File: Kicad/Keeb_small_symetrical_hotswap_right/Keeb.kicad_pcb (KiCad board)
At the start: 2 copper layers, 96.3 x 99.3 mm, 28 parts, among them J1 TYPE-C-31-M-12, SW1 CherryMX, SW10 CherryMX, SW11 CherryMX, SW13 CherryMX, SW14 CherryMX, SW15 CherryMX, SW16 CherryMX, SW17 CherryMX, SW18 CherryMX, SW19 CherryMX, SW20 CherryMX, SW3 CherryMX, SW4 CherryMX, SW5 CherryMX, SW6 CherryMX, SW7 CherryMX, SW8 CherryMX, SW9 CherryMX, U1 Pico

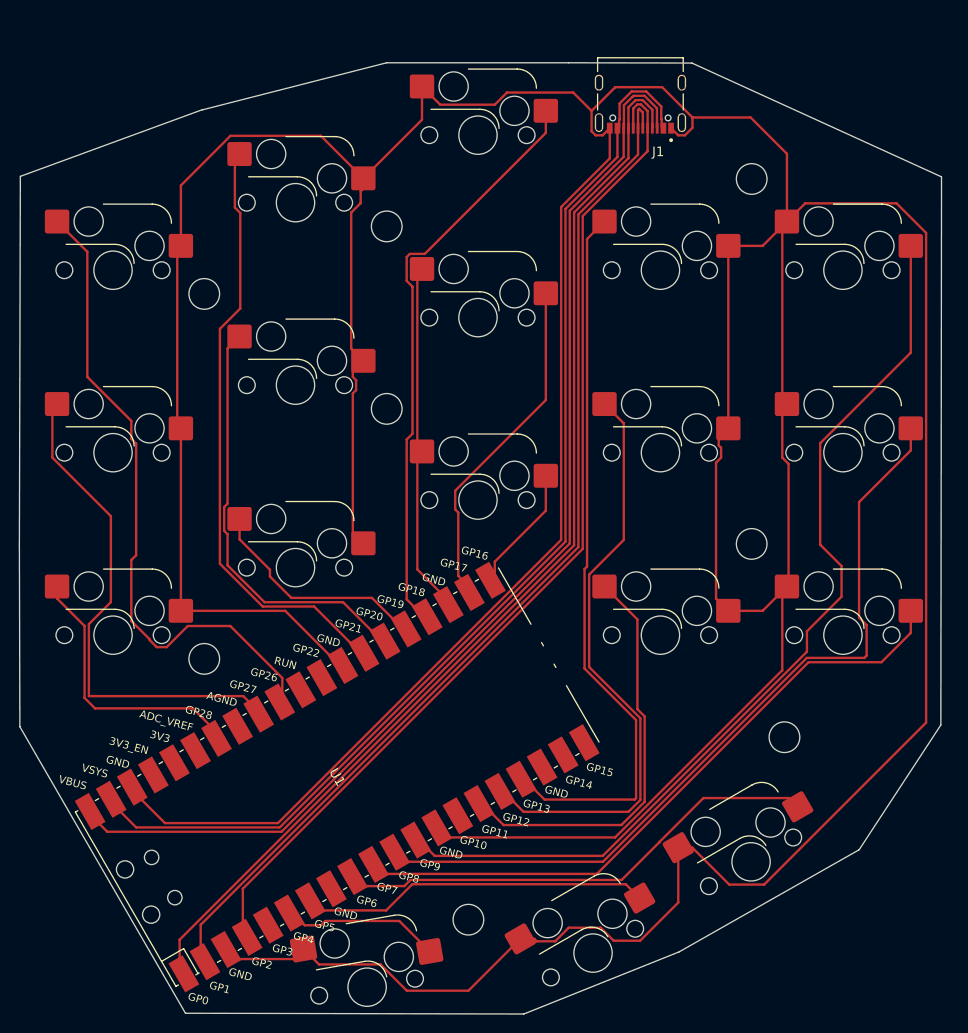
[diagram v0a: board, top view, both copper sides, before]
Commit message: Almost dome with right half
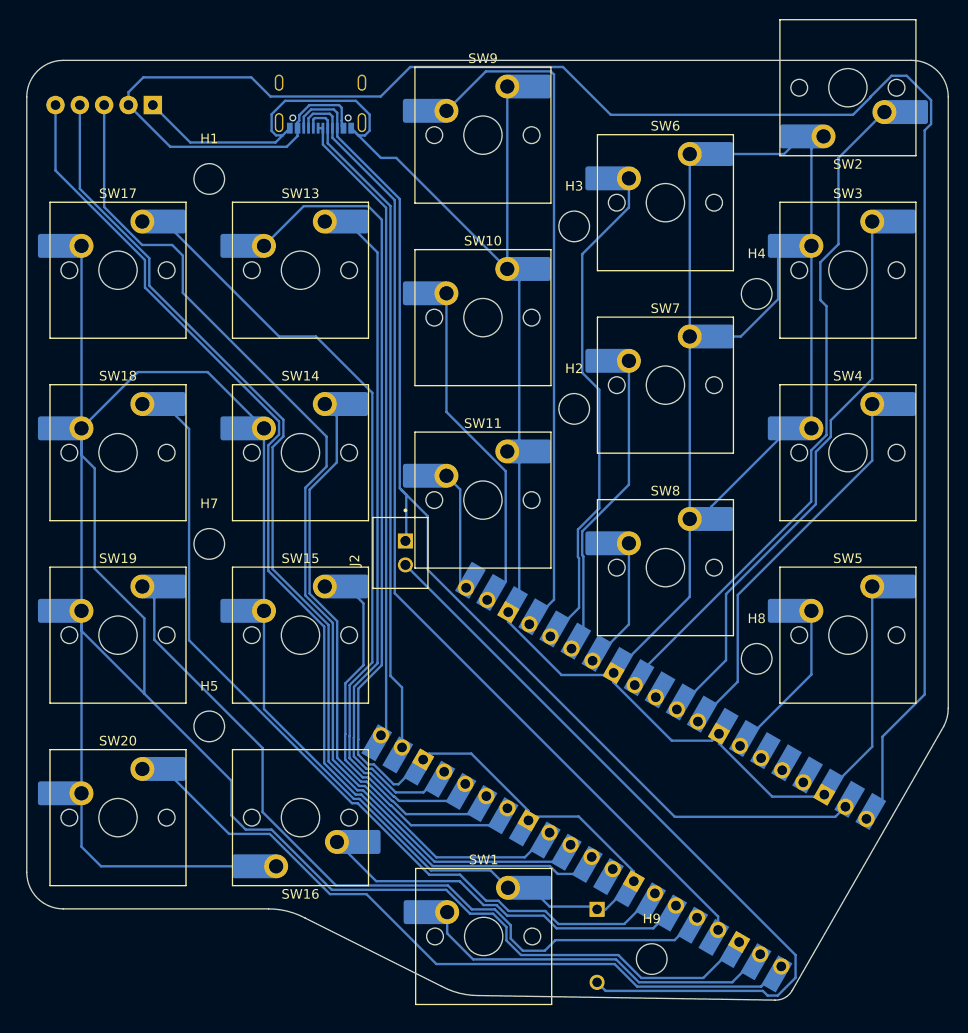
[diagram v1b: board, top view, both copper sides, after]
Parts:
- added J2: B2B-XH-A_LF__SN_, Connectors_user:JST_B2B-XH-A_LF__SN_, F.Cu at (141.6, 85.1)
- added S1: DS01-254-L-01BE, DIP:SW_DS01-254-L-01BE, B.Cu at (162.1, 126.2)
- added SW2: CherryMX, ScottoKeebs_Hotswap:Hotswap_MX_Plated_1.00u_Smaller_hole, F.Cu at (188.3, 36.6)
- added U2: KY-040, KY-040:KY-040-PORT, B.Cu at (110.7, 38.4)
- H1, H2, H3, H4, H5, H7, H8, H9: moved to F.Cu
- J1: moved to B.Cu
- SW1, SW10, SW11, SW13, SW14, SW15, SW16, SW17, SW18, SW19, SW20, SW3, SW4, SW5, SW6, SW7, SW8, SW9: footprint ScottoKeebs_Hotswap:Hotswap_MX_1.00u -> ScottoKeebs_Hotswap:Hotswap_MX_Plated_1.00u_Smaller_hole; moved to F.Cu
- U1: footprint MCU_RaspberryPi_and_Boards:RPi_Pico_SMD_TH_NO_HOLES -> MCU_RaspberryPi_and_Boards:RPi_Pico_SMD_TH_NO_BACK_HOLES; moved to B.Cu
- moved SW3 76.7 mm to (188.3, 55.6), turned to 0 degrees
- moved SW4 76.7 mm to (188.3, 74.7), turned to 0 degrees
- moved SW5 76.7 mm to (188.3, 93.7), turned to 0 degrees
- moved SW17 75.7 mm to (112.1, 55.6), turned to 0 degrees
- moved SW18 75.7 mm to (112.1, 74.7), turned to 0 degrees
- moved SW19 75.7 mm to (112.1, 93.7), turned to 0 degrees
- moved SW20 66.3 mm to (112.1, 112.8), turned to 0 degrees
- moved H5 60.1 mm to (121.7, 103.2), turned to 0 degrees
- moved H4 57.7 mm to (178.8, 58.1), turned to 0 degrees
- moved H8 57.7 mm to (178.8, 96.2), turned to 0 degrees
- moved H1 56.6 mm to (121.7, 46.1), turned to 0 degrees
- moved H7 56.6 mm to (121.7, 84.2), turned to 0 degrees
- moved SW6 38.6 mm to (169.3, 48.6), turned to 0 degrees
- moved SW7 38.6 mm to (169.3, 67.6), turned to 0 degrees
- moved SW8 38.6 mm to (169.3, 86.7), turned to 0 degrees
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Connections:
- J1 pad A4_B9: VSYS -> 3v3
- J1 pad A5: 0 -> 2
- J1 pad A6: 1 -> 15
- J1 pad A7: 1 -> 15
- J1 pad A8: 0 -> 2
- J1 pad B4_A9: VSYS -> 3v3
- J1 pad B5: 3v3 -> VSYS
- J1 pad B6: 2 -> 14
- J1 pad B7: 2 -> 14
- J1 pad B8: 3v3 -> VSYS
- SW1 pad 1: 4 -> 1
- SW14 pad 2: 12 -> 10
- SW16 pad 1: 5 -> 4
- SW17 pad 1: 9 -> GND
- SW17 pad 2: GND -> 12
- SW18 pad 1: 8 -> GND
- SW18 pad 2: GND -> 5
- SW19 pad 1: 7 -> GND
- SW19 pad 2: GND -> 3
- SW20 pad 1: 6 -> GND
- SW20 pad 2: GND -> 0
- SW5 pad 1: GND -> 28
- SW5 pad 2: 28 -> GND
- SW6 pad 1: GND -> 19
- SW6 pad 2: 21 -> GND
- SW7 pad 1: GND -> 20
- SW7 pad 2: 20 -> GND
- SW8 pad 1: GND -> 21
- SW8 pad 2: 19 -> GND
- U1 pad 33: unconnected-(U1-AGND-Pad33) -> GND
- U1 pad 8: unconnected-(U1-GND-Pad8) -> GND
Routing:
- net 3v3: track 117.2 -> 199.9 mm
- net Net-(J2-Pad2): track 0.00 -> 82.6 mm
- net 3: track 0.00 -> 82.3 mm
- net 14: track 0.00 -> 71.3 mm
- net 1: track 109.4 -> 38.2 mm
- net 22: track 0.00 -> 71.2 mm
- net GND: track 650.7 -> 719.6 mm
- net 15: track 0.00 -> 66.8 mm
- net 10: track 0.00 -> 61.2 mm
- net 6: track 51.9 -> 0.00 mm
- net 5: track 37.3 -> 88.0 mm
- net 21: track 63.8 -> 13.8 mm
- net 7: track 70.0 -> 114.7 mm
- net 0: track 114.3 -> 74.7 mm
- net 19: track 24.6 -> 52.8 mm
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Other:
- board size 96.3 x 99.3 mm -> 96.2 x 98.1 mm

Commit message: Fixedright board
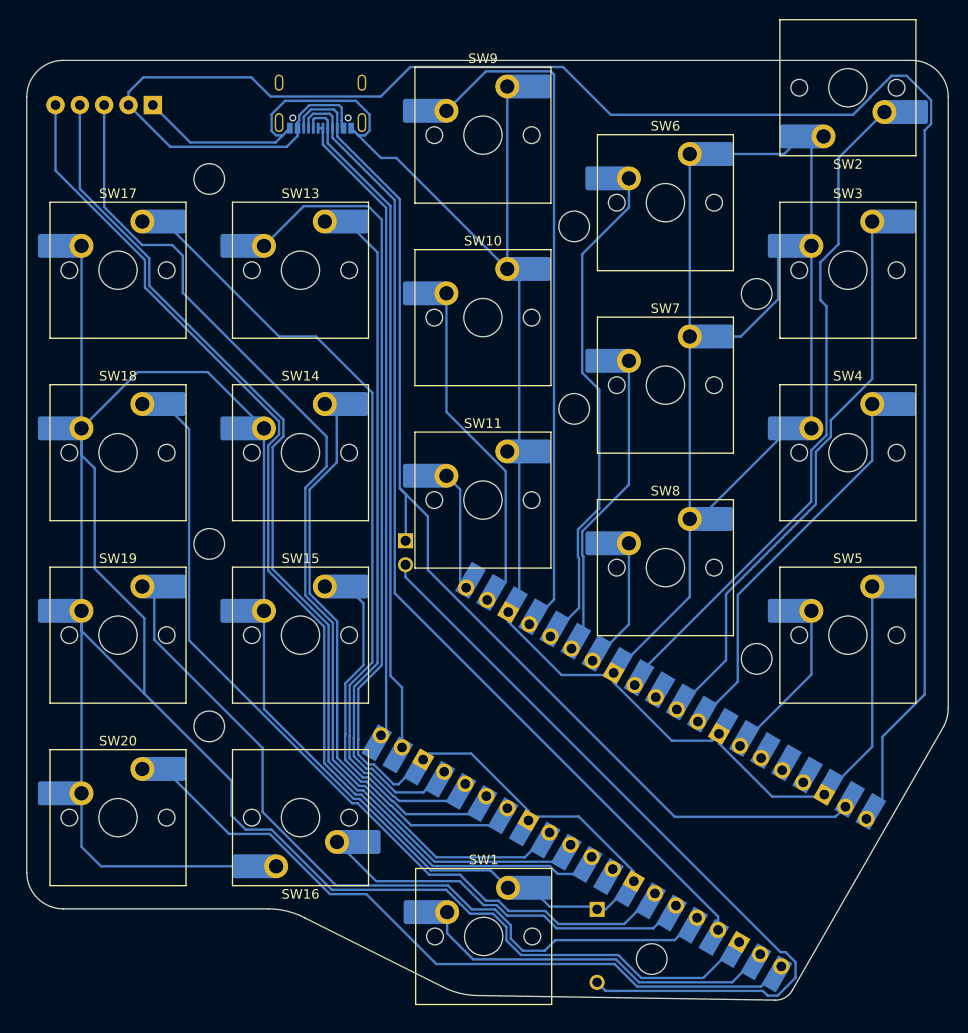
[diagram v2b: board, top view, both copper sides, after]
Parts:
- H1, H2, H3, H4, H5, H7, H8, H9, J2: moved to B.Cu
- moved J2 1.07 mm to (142.7, 85.1)
- turned H1 to 180 degrees
- turned H2 to 180 degrees
- turned H3 to 180 degrees
- turned H4 to 180 degrees
- turned H5 to 180 degrees
- turned H7 to 180 degrees
- turned H8 to 180 degrees
- turned H9 to 180 degrees
